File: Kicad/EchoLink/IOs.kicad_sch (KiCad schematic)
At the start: 5 parts, among them J3 Conn_01x08_Pin, J4 Conn_01x06_Pin, J5 Conn_01x09_Socket

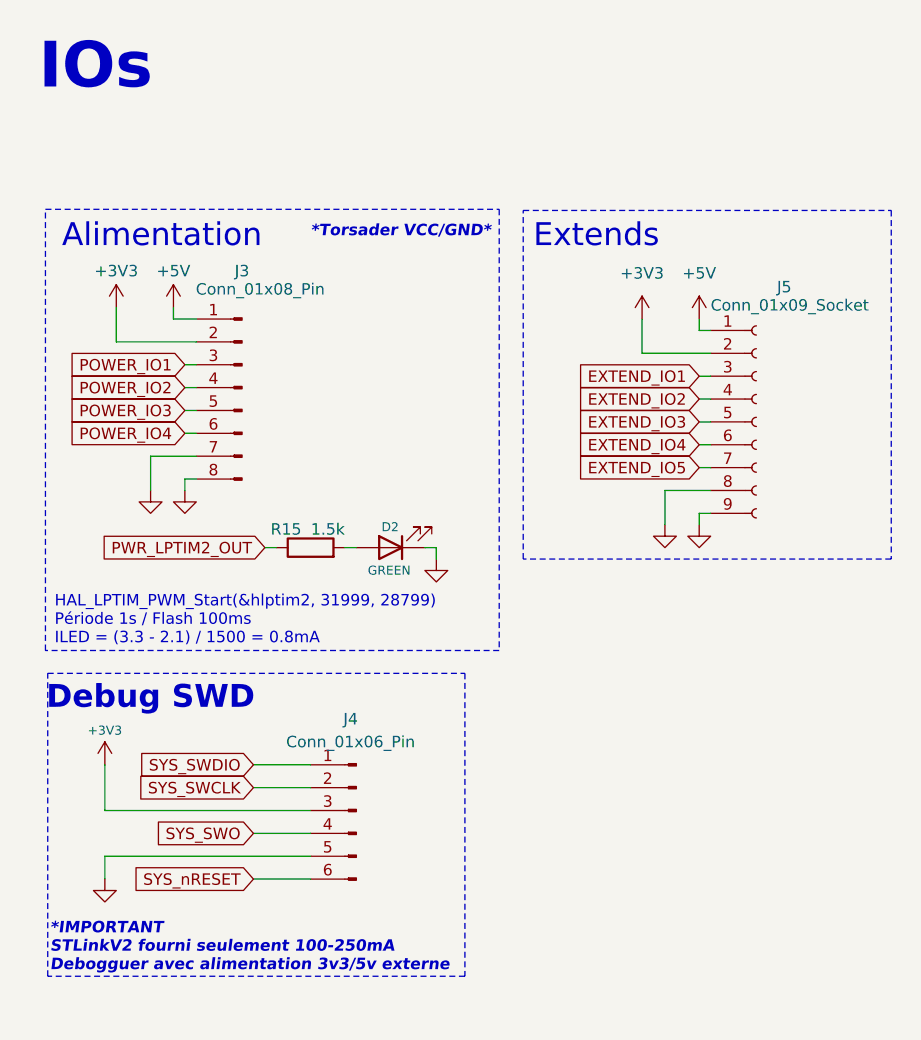
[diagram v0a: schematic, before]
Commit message: wip: connector and bms IOs
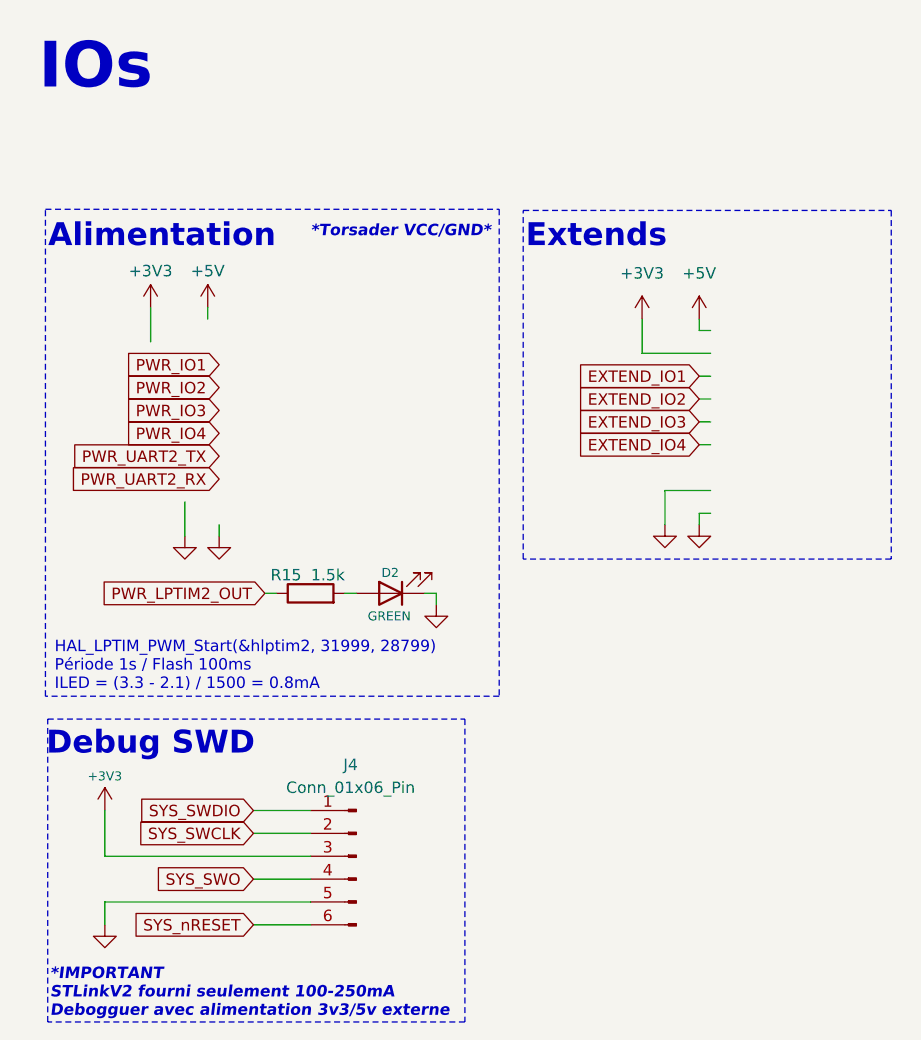
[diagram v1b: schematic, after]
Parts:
- removed J3: Conn_01x08_Pin, symbol Connector:Conn_01x08_Pin
- removed J5: Conn_01x09_Socket, symbol Connector:Conn_01x09_Socket
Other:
- moved on the sheet: D2, J4, R15
